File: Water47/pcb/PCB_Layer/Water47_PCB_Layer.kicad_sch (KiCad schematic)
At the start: 104 parts, among them SW1 Esc, SW10 O, SW11 P, SW12 -, SW13 Del, SW14 Cmd, SW15 A, SW16 S, SW17 D, SW18 F, SW19 G, SW2 Q, SW20 H, SW21 J, SW22 K, SW23 L, SW24 ;, SW25 Bs, SW26 Shift(L), SW27 Z, SW28 X, SW29 C, SW3 W, SW30 V, SW31 B, SW32 N, SW33 M, SW34 ,, SW35 ., SW36 Shift(R), SW37 Fn, SW38 Ctrl(L), SW39 Win(L), SW4 E, SW40 Alt(L), SW41 Shift(C), SW42 Fn(C), SW43 Enter, SW44 ←, SW45 ↓, SW46 ↑, SW47 →, SW5 R, SW6 T, SW7 Y, SW8 U, SW9 I, U1 MOUDLE-SEEEDUINO-XIAO

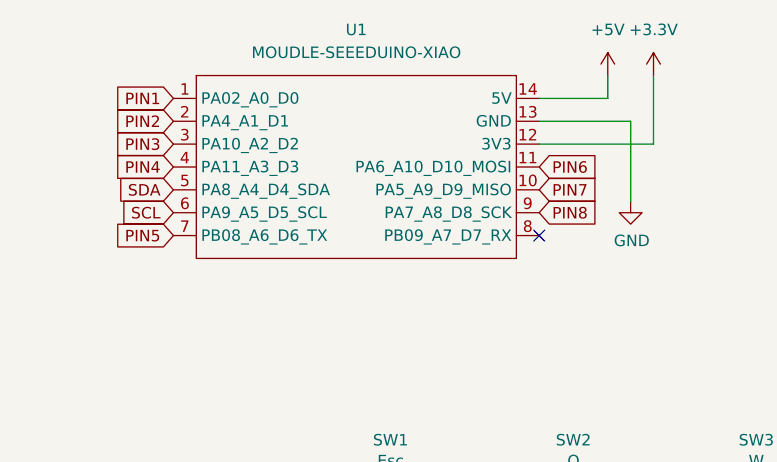
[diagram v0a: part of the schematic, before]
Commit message: feat: first wiring
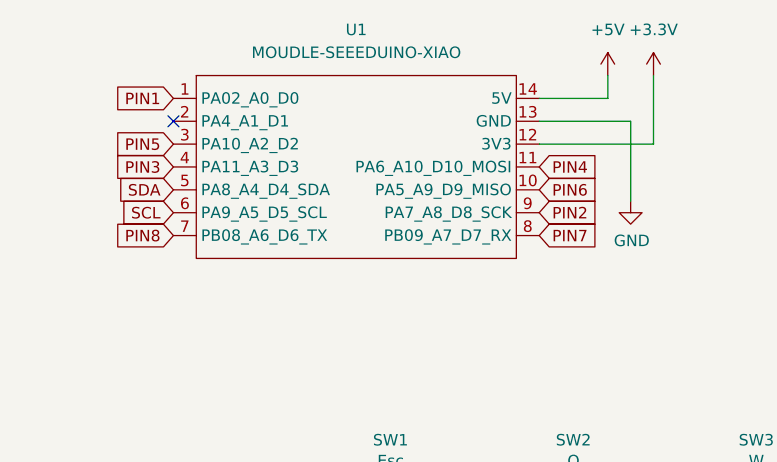
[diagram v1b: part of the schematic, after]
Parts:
- SW1, SW10, SW11, SW12, SW13, SW15, SW16, SW17, SW18, SW19, SW2, SW20, SW21, SW22, SW23, SW24, SW27, SW28, SW29, SW3, SW30, SW31, SW32, SW33, SW34, SW35, SW37, SW4, SW44, SW45, SW46, SW47, SW5, SW6, SW7, SW8, SW9: footprint multifeb13_kbd_KiCad_lib:Kailh_Choc_V1_Hotswap_via_1u -> multifeb13_kbd_KiCad_lib:Kailh_Choc_V2_1u_wo_anker
- SW14, SW36, SW38, SW39, SW40, SW42: footprint multifeb13_kbd_KiCad_lib:Kailh_Choc_V1_Hotswap_via_1.25u -> multifeb13_kbd_KiCad_lib:Kailh_Choc_V2_1.25u_wo_anker
- SW25, SW26: footprint multifeb13_kbd_KiCad_lib:Kailh_Choc_V1_Hotswap_via_1.75u -> multifeb13_kbd_KiCad_lib:Kailh_Choc_V2_1.75u_wo_anker
- SW41, SW43: footprint multifeb13_kbd_KiCad_lib:Kailh_Choc_V1_Hotswap_via_2u -> multifeb13_kbd_KiCad_lib:Kailh_Choc_V2_2u_wo_anker
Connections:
- net PIN2: now also U1.9 (PA7_A8_D8_SCK); no longer U1.2 (PA4_A1_D1)
- net PIN3: now also U1.4 (PA11_A3_D3); no longer U1.3 (PA10_A2_D2)
- net PIN4: now also U1.11 (PA6_A10_D10_MOSI); no longer U1.4 (PA11_A3_D3)
- net PIN5: now also U1.3 (PA10_A2_D2); no longer U1.7 (PB08_A6_D6_TX)
- net PIN6: now also U1.10 (PA5_A9_D9_MISO); no longer U1.11 (PA6_A10_D10_MOSI)
- net PIN7: now also U1.8 (PB09_A7_D7_RX); no longer U1.10 (PA5_A9_D9_MISO)
- net PIN8: now also U1.7 (PB08_A6_D6_TX); no longer U1.9 (PA7_A8_D8_SCK)
